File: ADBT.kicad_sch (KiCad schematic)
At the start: 107 parts, among them J1 ADB1, J2 microUSB, J3 JTAG, Q1 AO3401, Q2 MMBT3904, Q3 MMBT3904, Q4 MMBT3904, Q5 MMBT3904, Q6 AO3401, Q7 AO3401, SW1 SW_Push, SW2 SW_Push, U1 ESP-WROOM-32, U2 CH340G, U3 MP2451DT, U4 74LVC1G14GW, Y1 12M

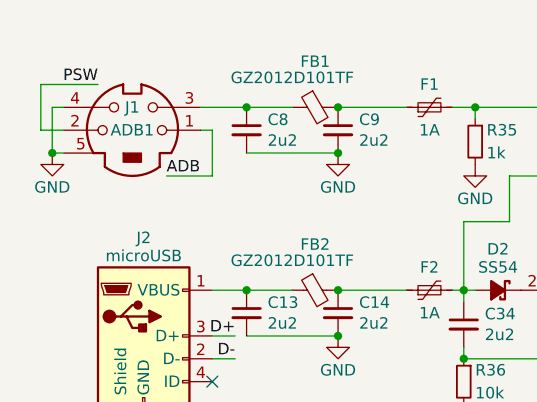
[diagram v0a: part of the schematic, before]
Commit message: idk
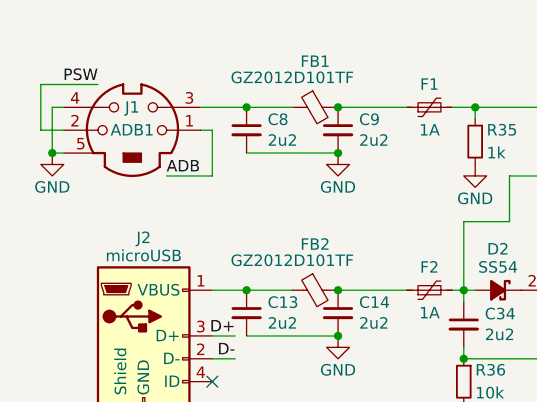
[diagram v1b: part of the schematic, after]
